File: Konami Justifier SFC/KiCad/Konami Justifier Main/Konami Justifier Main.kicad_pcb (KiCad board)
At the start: 4 copper layers, 25.2 x 50 mm, 20 parts, among them J1 RJ12, J2 Conn_01x06_Socket, U1 74VHC9164FT

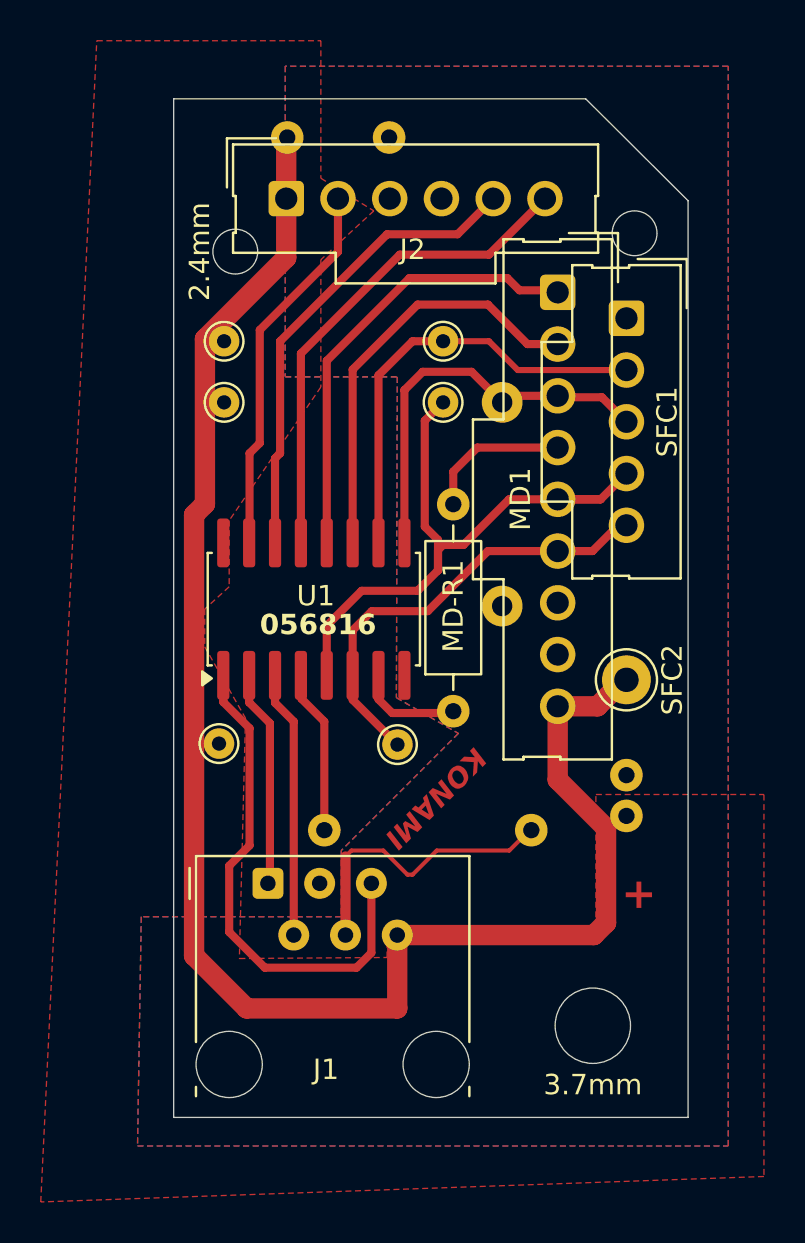
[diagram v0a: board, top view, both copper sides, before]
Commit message: Add files via upload
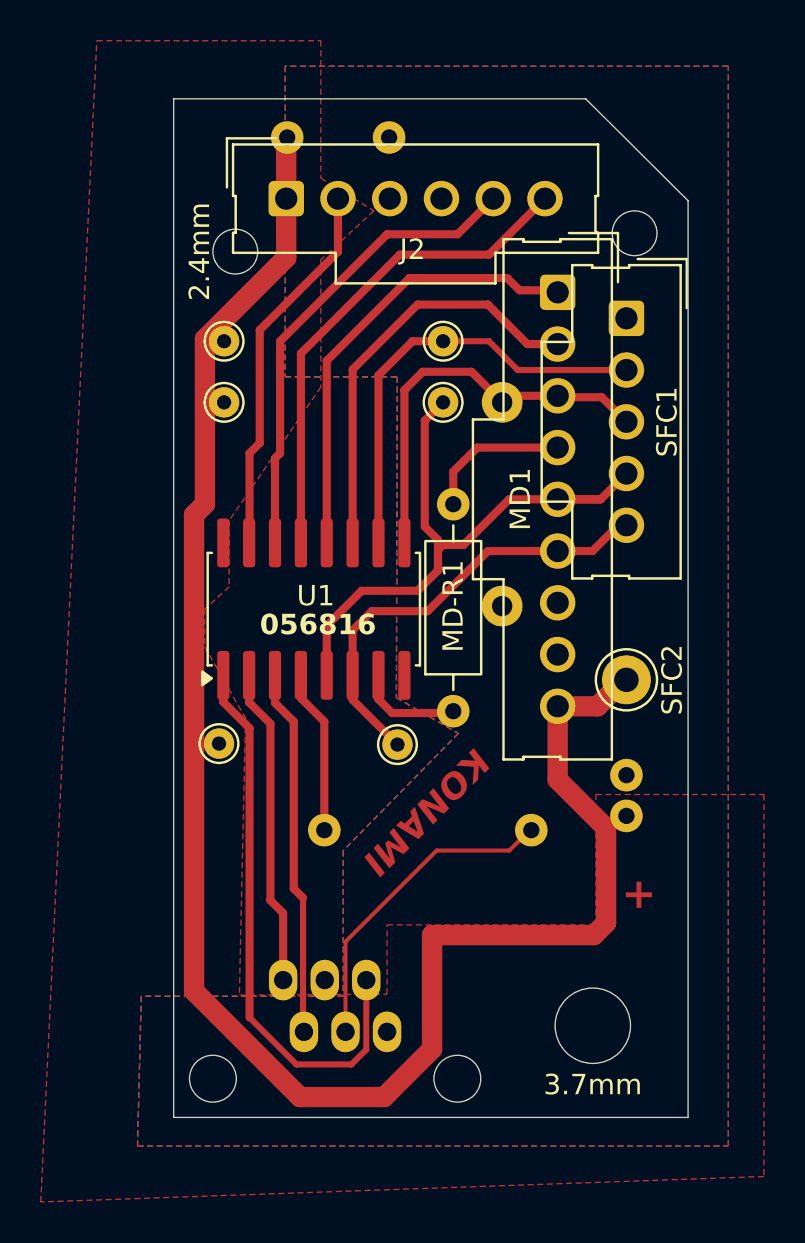
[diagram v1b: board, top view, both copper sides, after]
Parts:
- J1: footprint Connector_RJ:RJ12_Amphenol_54601-x06_Horizontal -> Connector_RJ:RJ25_Wayconn_MJEA-660X1_Horizontal; moved to B.Cu
- moved J1 4.81 mm to (145.2, 119.9), turned to 180 degrees
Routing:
- net +5V: track 82.8 -> 88.6 mm
- net Net-(U1-SI): track 13.1 -> 18.1 mm
- net Net-(U1-~{CLR_LOAD}): track 10.7 -> 15.7 mm
- net Net-(U1-P/S_CONT): track 25.0 -> 27.7 mm
- net GND: track 14.7 -> 16.0 mm

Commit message: Add files via upload
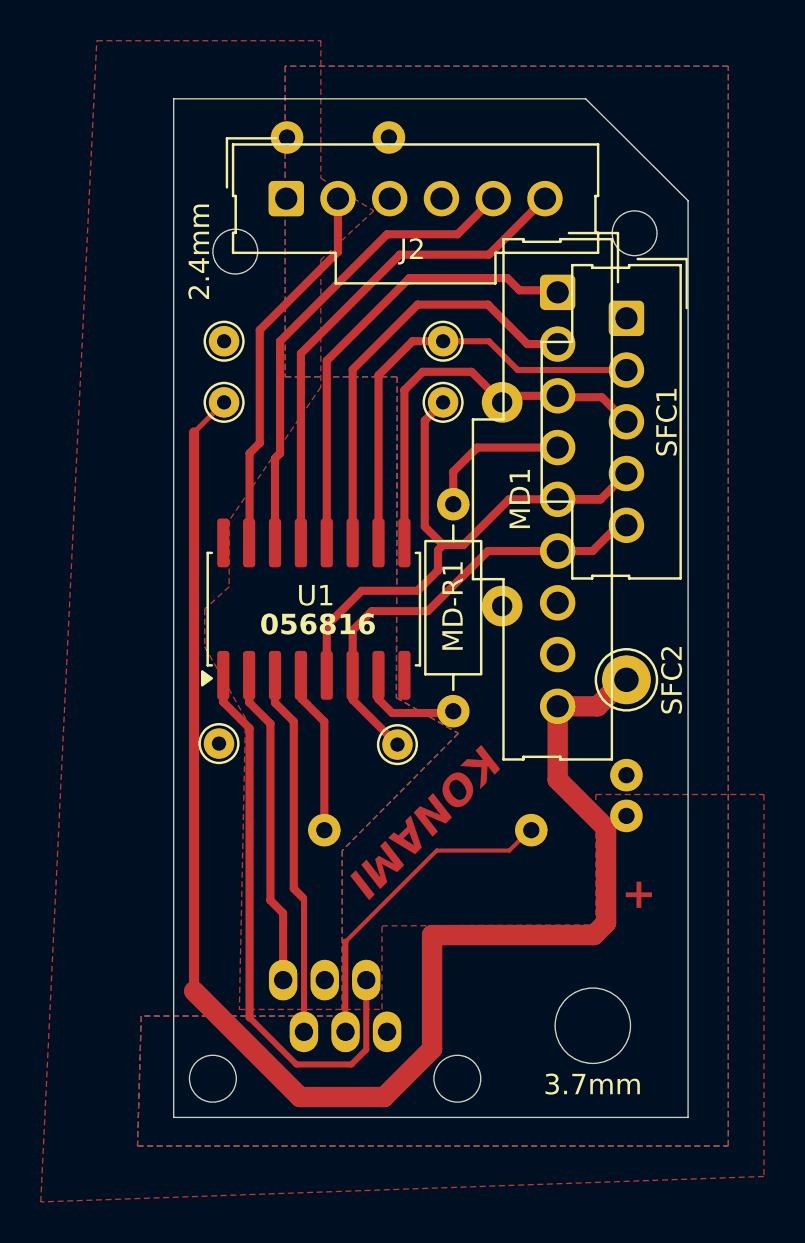
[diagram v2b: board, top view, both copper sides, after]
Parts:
- moved C2 5.01 mm to (145.3, 78.5), turned to 0 degrees
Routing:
- net +5V: track 88.6 -> 74.3 mm
- net Net-(MD1-Pin_5): track 32.1 -> 30.9 mm

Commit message: Add files via upload
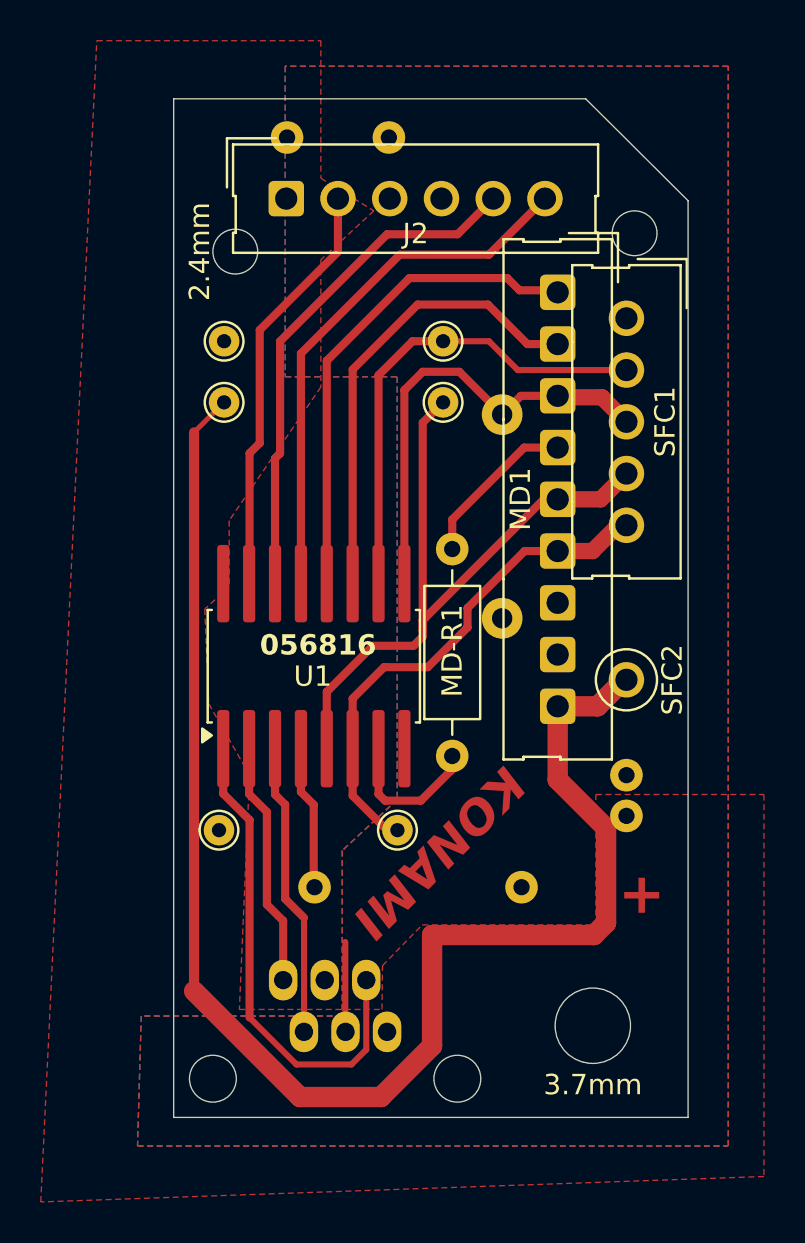
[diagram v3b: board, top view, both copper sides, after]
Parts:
- moved SFC-TP5 4.25 mm to (142.0, 112.5)
- moved SFC-TP6 4.20 mm to (150.8, 112.5)
- moved SFC-R1 2.84 mm to (156.8, 115.3)
- moved U1 2.80 mm to (146.7, 104.5)
- moved MD-R1 2.20 mm to (153.4, 108.9)
- moved SFC-C1 0.60 mm to (155.9, 92.1)
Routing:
- net GND: track 16.0 -> 4.42 mm
- net Net-(MD1-Pin_2): track 21.7 -> 27.3 mm
- net Net-(U1-Q/D3): track 5.16 -> 10.2 mm
- net Net-(MD1-Pin_5): track 30.9 -> 35.6 mm
- net Net-(MD1-Pin_6): track 22.4 -> 25.5 mm
- net Net-(U1-P/S_CONT): track 27.7 -> 24.9 mm
- net Net-(SFC1-Pin_2): track 21.7 -> 24.5 mm
- net Net-(MD1-Pin_1): track 22.2 -> 25.0 mm
- net Net-(J2-Pin_6): track 24.4 -> 27.2 mm
- net Net-(J2-Pin_5): track 23.4 -> 26.2 mm
- net Net-(J2-Pin_2): track 18.7 -> 21.5 mm
- net Net-(U1-~{CLR_LOAD}): track 15.7 -> 12.9 mm
- net Net-(U1-SI): track 18.1 -> 15.3 mm
- net Net-(MD1-Pin_3): track 21.6 -> 24.1 mm
- net Net-(MD1-Pin_4): track 7.21 -> 8.71 mm
